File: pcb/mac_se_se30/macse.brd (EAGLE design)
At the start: 52 x 24 mm, 8 parts, among them J1 ATX24RH

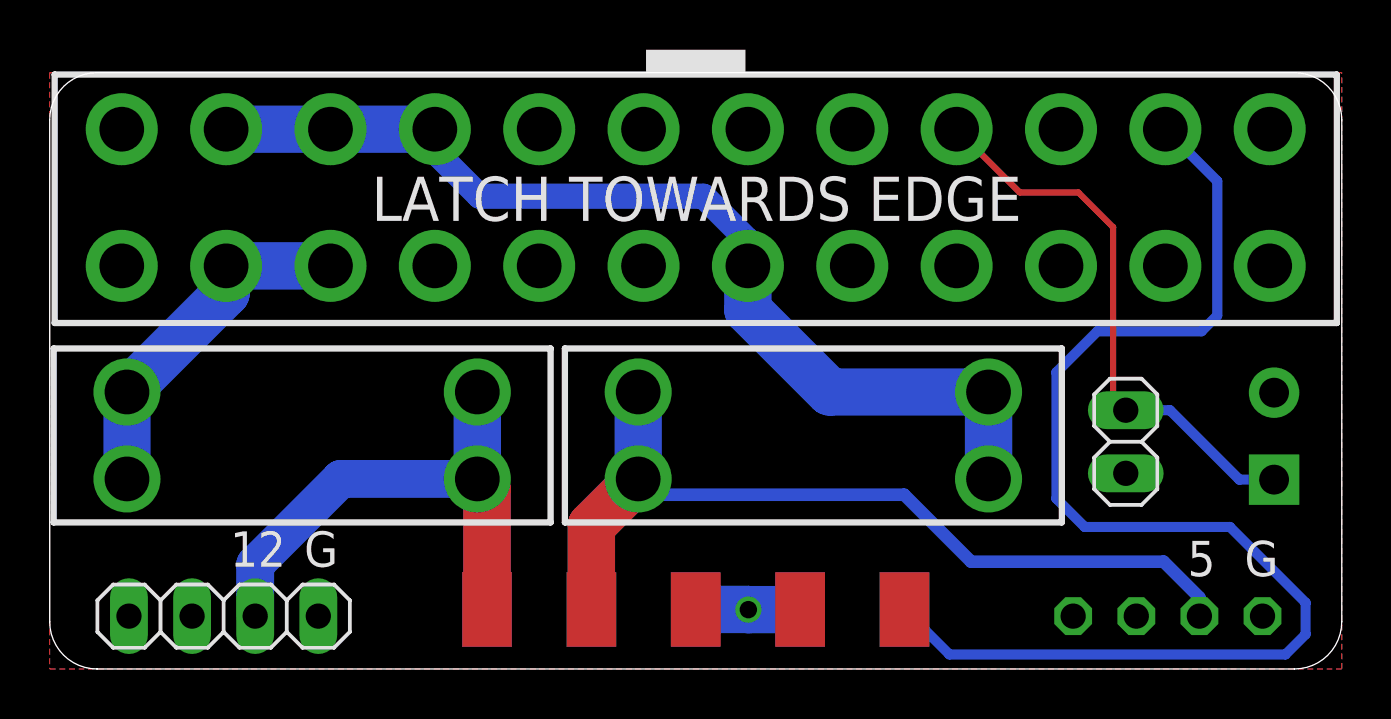
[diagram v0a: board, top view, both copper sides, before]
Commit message: mac SE adaptor done
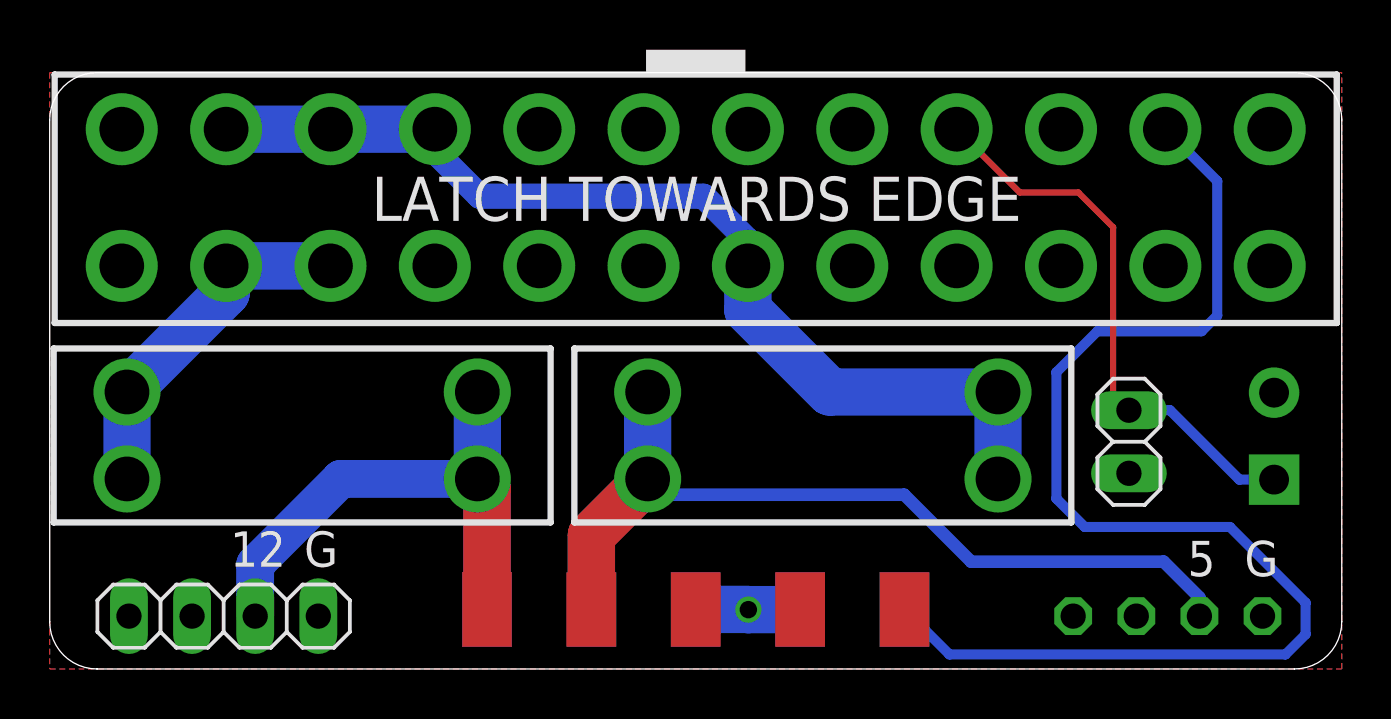
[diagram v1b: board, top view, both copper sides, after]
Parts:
- moved U$8 0.38 mm to (31.1, 9.40)
- moved JP2 0.13 mm to (43.4, 9.14)
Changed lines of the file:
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@@
 <attribute name="VALUE" x="42.46" y="-1.048" size="1.27" layer="27"/>
 </element>
-<element name="U$8" library="atx_power_control" package="FUSE_HOLDER_3IN1" value="CAR_FUSE_HOLDER3IN1" x="30.734" y="9.398" smashed="yes"/>
+<element name="U$8" library="atx_power_control" package="FUSE_HOLDER_3IN1" value="CAR_FUSE_HOLDER3IN1" x="31.115" y="9.398" smashed="yes"/>
 <element name="U$2" library="atx_power_control" package="FUSE_HOLDER_3IN1" value="CAR_FUSE_HOLDER3IN1" x="10.16" y="9.398" smashed="yes"/>
-<element name="JP2" library="pinhead" library_urn="urn:adsk.eagle:library:325" package="1X02" package3d_urn="urn:adsk.eagle:package:22435/2" value="" x="43.307" y="9.144" smashed="yes" rot="R270">
-<attribute name="POPULARITY" value="98" x="43.307" y="9.144" size="1.778" layer="27" rot="R270" display="off"/>
-<attribute name="VALUE" x="40.132" y="11.684" size="1.27" layer="27" rot="R270"/>
+<element name="JP2" library="pinhead" library_urn="urn:adsk.eagle:library:325" package="1X02" package3d_urn="urn:adsk.eagle:package:22435/2" value="" x="43.434" y="9.144" smashed="yes" rot="R270">
+<attribute name="POPULARITY" value="98" x="43.434" y="9.144" size="1.778" layer="27" rot="R270" display="off"/>
+<attribute name="VALUE" x="40.259" y="11.684" size="1.27" layer="27" rot="R270"/>
 </element>
 <element name="U$1" library="atx4vc" package="MACSE_10P" value="MACSE" x="26" y="2.394" smashed="yes" rot="MR180"/>
@@
 <contactref element="U$1" pad="P$9"/>
 <contactref element="JP4" pad="3"/>
-<wire x1="23.684" y1="11.148" x2="23.684" y2="7.648" width="1.905" layer="16"/>
-<wire x1="23.684" y1="7.648" x2="21.8" y2="5.764" width="1.905" layer="16"/>
-<wire x1="21.8" y1="5.764" x2="21.8" y2="2.394" width="1.905" layer="16"/>
+<wire x1="24.065" y1="11.148" x2="24.065" y2="7.648" width="1.905" layer="16"/>
+<wire x1="24.065" y1="7.648" x2="21.8" y2="5.383" width="1.905" layer="16"/>
+<wire x1="21.8" y1="5.383" x2="21.8" y2="2.394" width="1.905" layer="16"/>
 <wire x1="46.27" y1="2.127" x2="46.27" y2="2.879" width="0.508" layer="16"/>
 <wire x1="46.27" y1="2.879" x2="44.831" y2="4.318" width="0.508" layer="16"/>
 <wire x1="44.831" y1="4.318" x2="37.084" y2="4.318" width="0.508" layer="16"/>
-<wire x1="34.389" y1="7.013" x2="24.319" y2="7.013" width="0.508" layer="16"/>
-<wire x1="24.319" y1="7.013" x2="23.684" y2="7.648" width="0.508" layer="16"/>
+<wire x1="34.389" y1="7.013" x2="24.7" y2="7.013" width="0.508" layer="16"/>
+<wire x1="24.7" y1="7.013" x2="24.065" y2="7.648" width="0.508" layer="16"/>
 <wire x1="37.084" y1="4.318" x2="34.389" y2="7.013" width="0.508" layer="16"/>
-<wire x1="23.684" y1="7.648" x2="21.8" y2="5.764" width="1.905" layer="1"/>
-<wire x1="21.8" y1="5.764" x2="21.8" y2="2.394" width="1.905" layer="1"/>
+<wire x1="24.065" y1="7.648" x2="21.8" y2="5.383" width="1.905" layer="1"/>
+<wire x1="21.8" y1="5.383" x2="21.8" y2="2.394" width="1.905" layer="1"/>
 </signal>
 <signal name="-12V">
@@
 <wire x1="26.3144" y1="19.0246" x2="28.1" y2="17.239" width="1.016" layer="16"/>
 <wire x1="28.1" y1="16.223" x2="28.1" y2="14.445" width="1.905" layer="16"/>
-<wire x1="31.397" y1="11.148" x2="37.784" y2="11.148" width="1.905" layer="16"/>
+<wire x1="31.397" y1="11.148" x2="38.165" y2="11.148" width="1.905" layer="16"/>
 <wire x1="28.1" y1="14.445" x2="31.397" y2="11.148" width="1.905" layer="16"/>
-<wire x1="37.784" y1="11.148" x2="37.784" y2="7.648" width="1.905" layer="16"/>
+<wire x1="38.165" y1="11.148" x2="38.165" y2="7.648" width="1.905" layer="16"/>
 </signal>
 <signal name="N$8">
@@
 <wire x1="39.046" y1="19.177" x2="41.402" y2="19.177" width="0.254" layer="1"/>
 <wire x1="41.402" y1="19.177" x2="42.799" y2="17.78" width="0.254" layer="1"/>
-<wire x1="42.799" y1="10.922" x2="43.307" y2="10.414" width="0.254" layer="1"/>
-<wire x1="42.799" y1="17.78" x2="42.799" y2="10.922" width="0.254" layer="1"/>
-<wire x1="43.307" y1="10.414" x2="45.085" y2="10.414" width="0.4064" layer="16"/>
+<wire x1="42.799" y1="11.049" x2="43.434" y2="10.414" width="0.254" layer="1"/>
+<wire x1="42.799" y1="17.78" x2="42.799" y2="11.049" width="0.254" layer="1"/>
+<wire x1="43.434" y1="10.414" x2="45.085" y2="10.414" width="0.4064" layer="16"/>
 <wire x1="47.879" y1="7.62" x2="49.276" y2="7.62" width="0.4064" layer="16"/>
 <wire x1="45.085" y1="10.414" x2="47.879" y2="7.62" width="0.4064" layer="16"/>
